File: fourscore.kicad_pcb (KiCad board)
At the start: 2 copper layers, 138 x 43 mm, 33 parts, among them J1 Conn_01x07_Socket, J2 Conn_01x07_Socket, J3 Conn_01x07_Socket, J4 Conn_01x07_Socket, J5 Conn_01x07_Socket, SW1 2-4, SW2 B, SW3 A

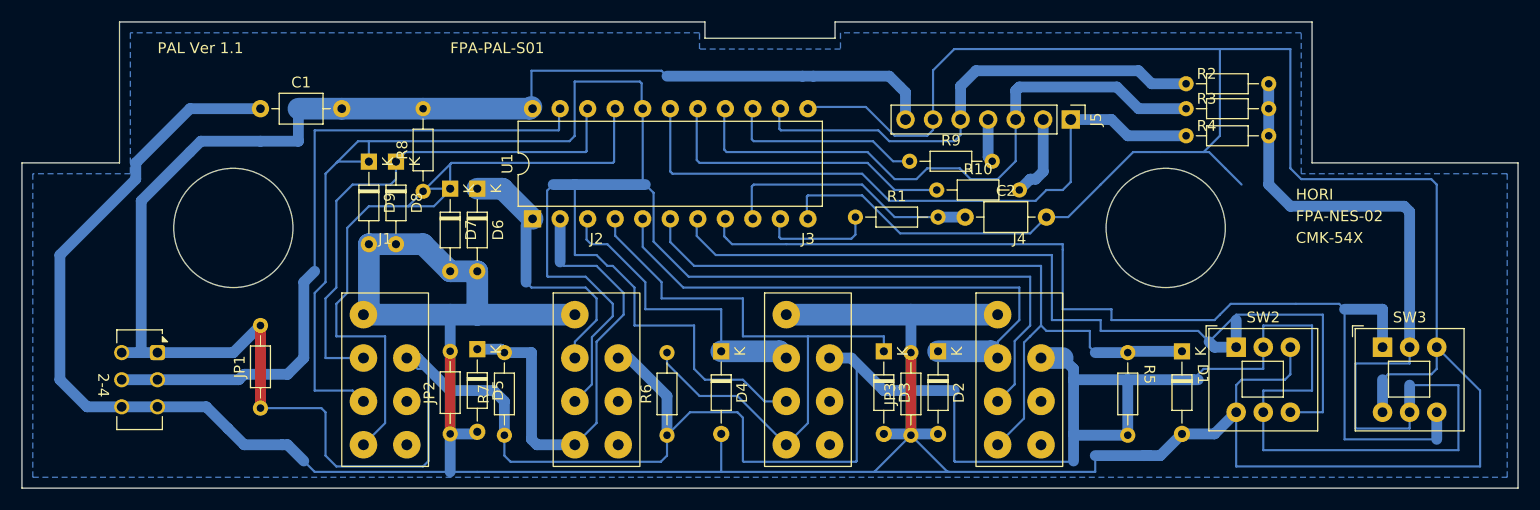
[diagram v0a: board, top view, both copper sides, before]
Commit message: dealt with all warnings
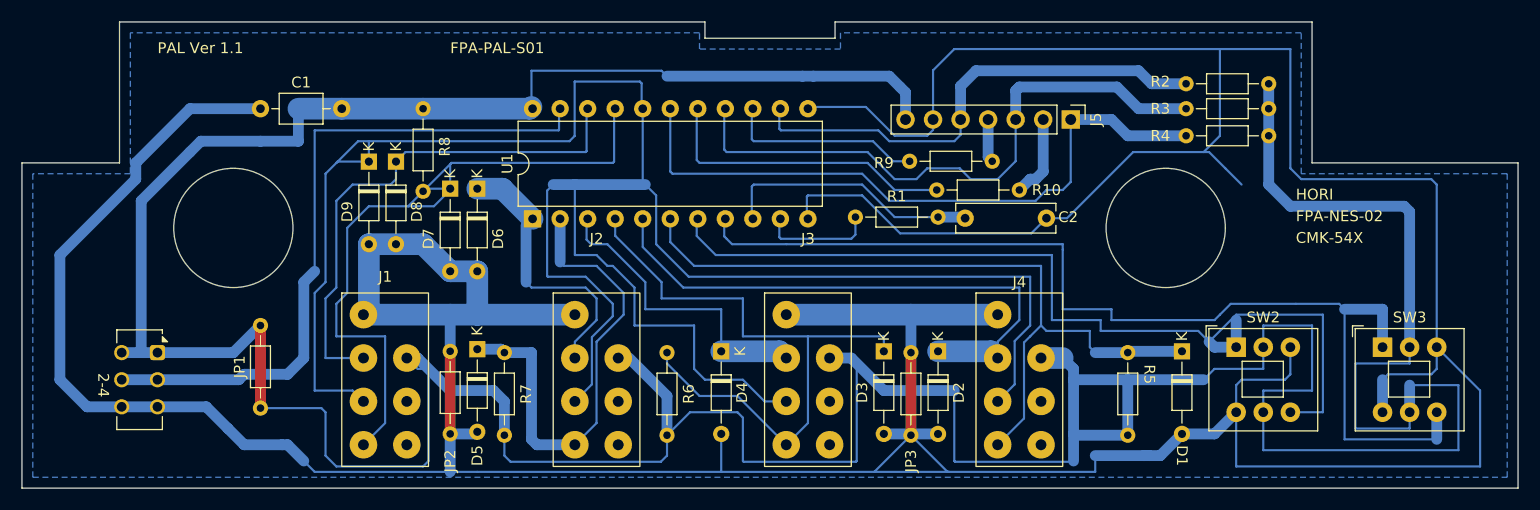
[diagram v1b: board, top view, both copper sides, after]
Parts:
- C2: footprint Capacitor_THT:C_Axial_L3.8mm_D2.6mm_P7.50mm_Horizontal -> Capacitor_THT:C_Rect_L9.0mm_W2.5mm_P7.50mm_MKT
- moved C2 0.10 mm to (177.0, 78.1)
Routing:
- net VCC: track 407.2 -> 406.7 mm
